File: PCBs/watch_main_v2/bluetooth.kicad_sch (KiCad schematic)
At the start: 24 parts, among them U301 NRF5340-QKAA-R7, Y301 32MHz

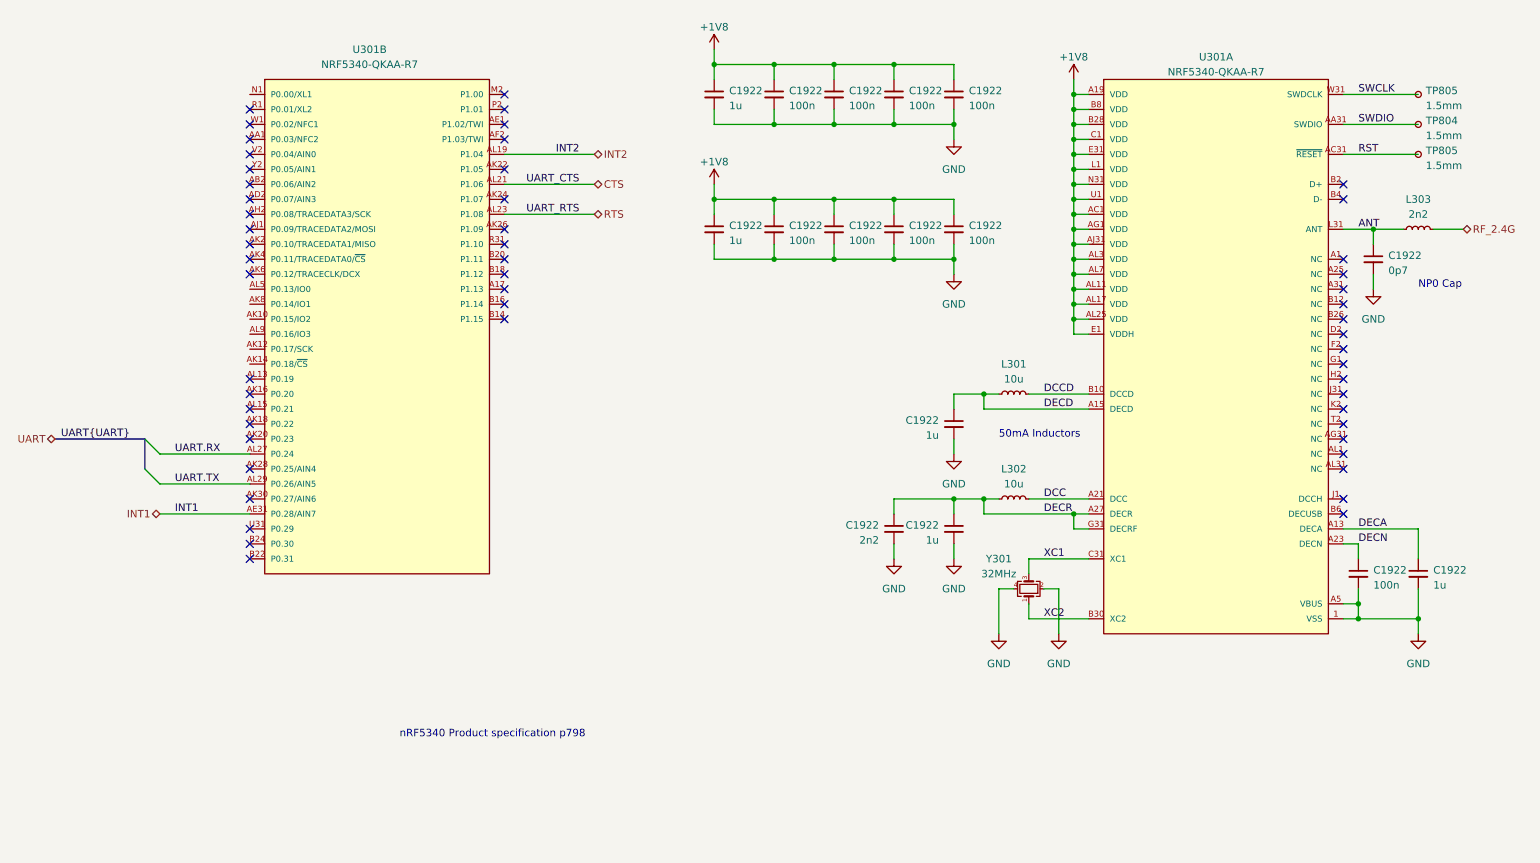
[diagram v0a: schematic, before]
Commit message: Schematic v2 complete
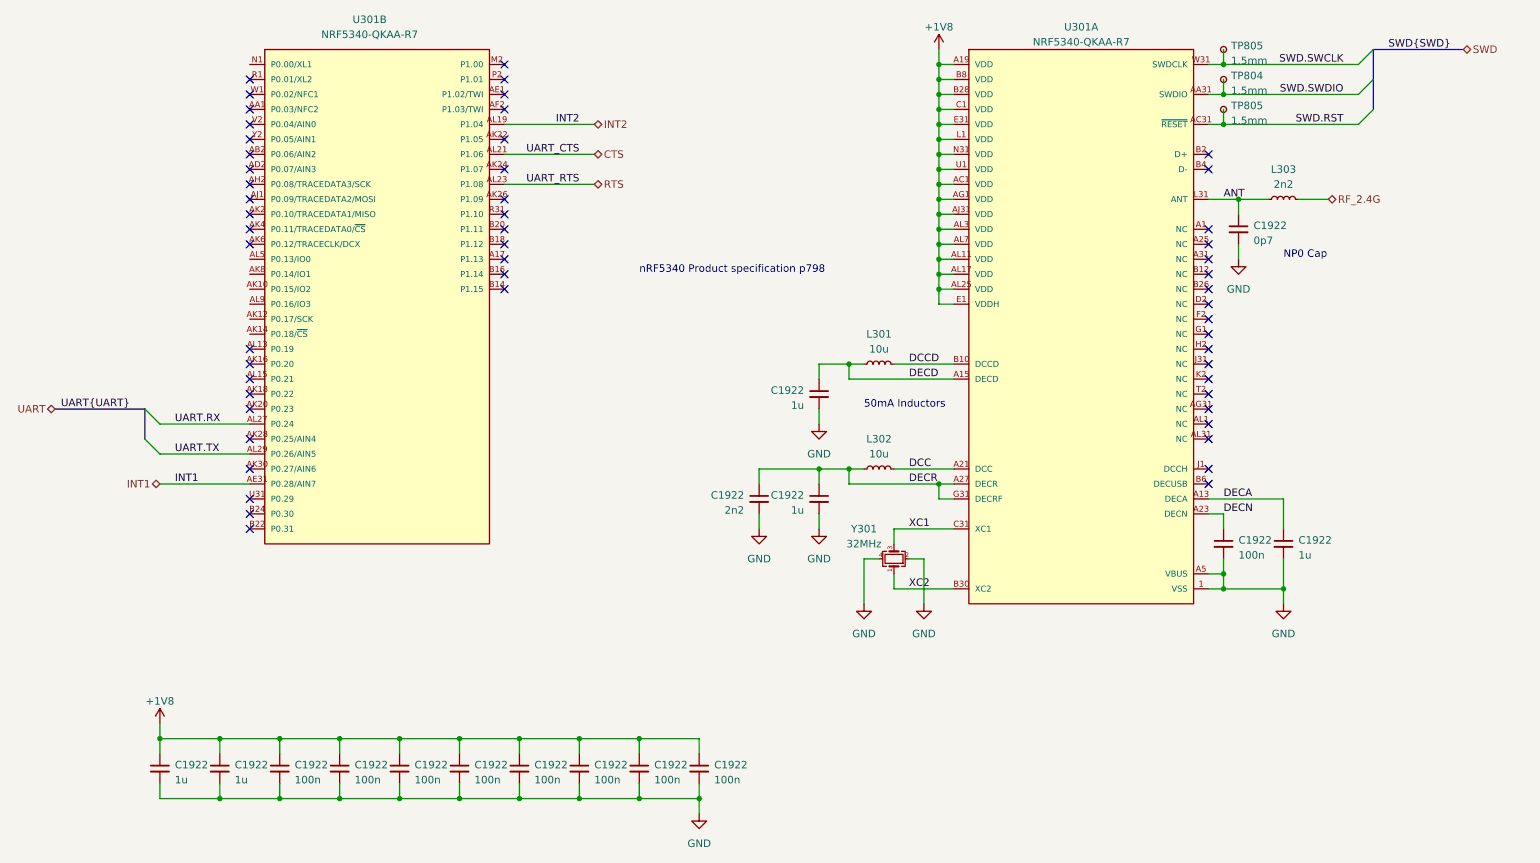
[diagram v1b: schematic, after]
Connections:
- net RST renamed SWD.RST
- net SWCLK renamed SWD.SWCLK
- net SWDIO renamed SWD.SWDIO
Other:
- moved on the sheet: C1922, L301, L302, L303, TP804, TP805, U301A, U301B, Y301
